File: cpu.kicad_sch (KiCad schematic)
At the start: 41 parts, among them J11 Debug, J12 GPS_Snoop, J13 I2C_Snoop, J6 USB_C_Receptacle_16P, SW1 Reset, U4 STM32H503KBUx, Y1 32768Hz

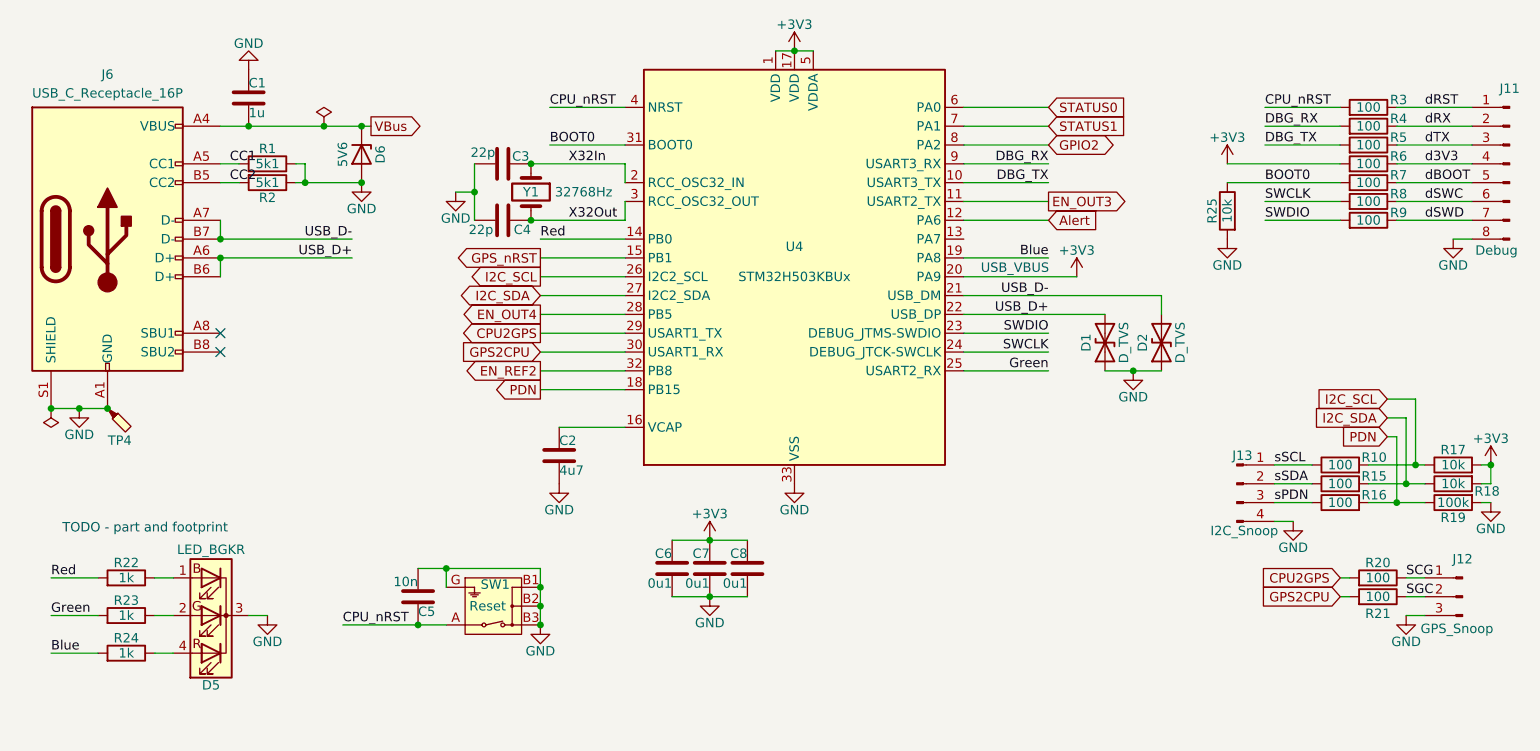
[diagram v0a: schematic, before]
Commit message: Placement looks sane.
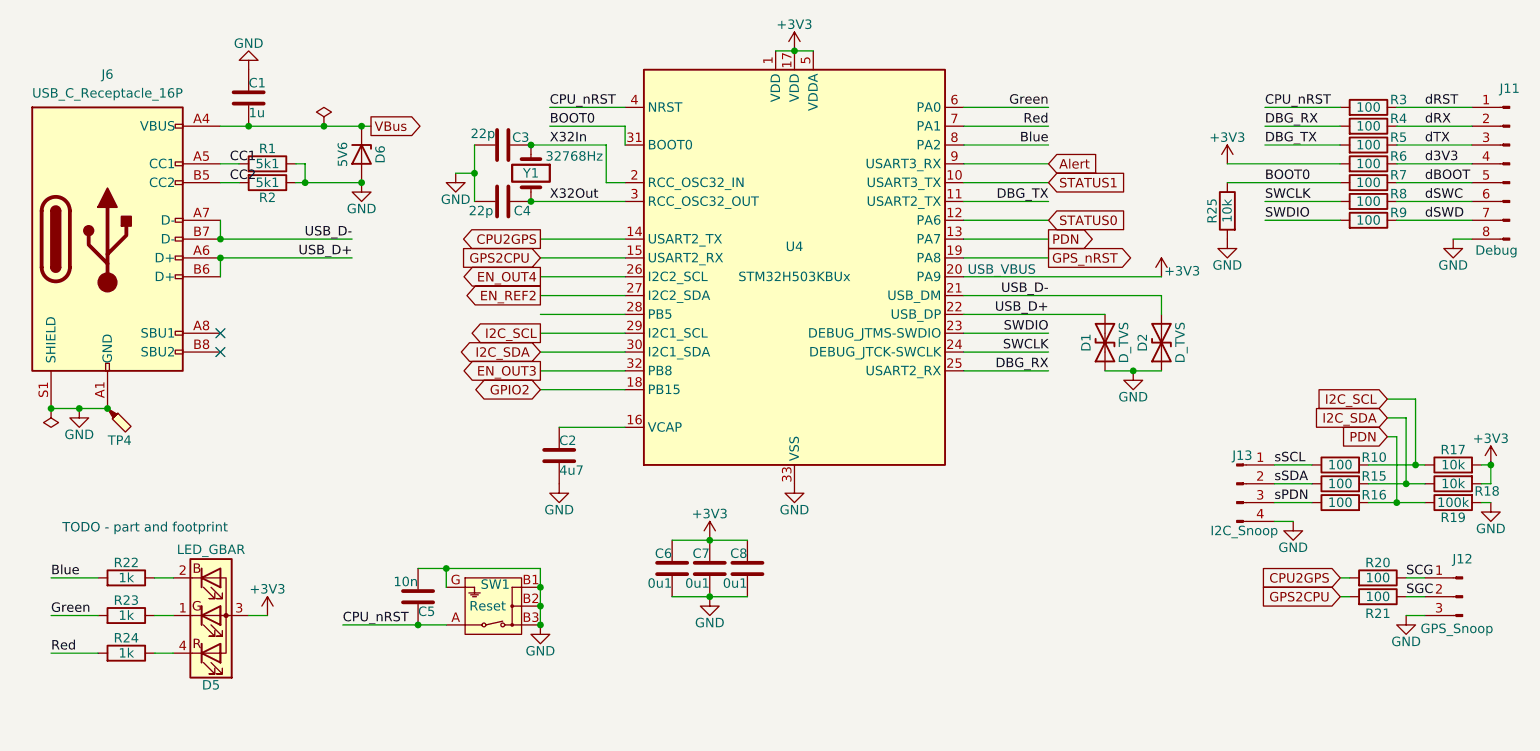
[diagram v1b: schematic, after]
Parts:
- D5: value LED_BGKR -> LED_GBAR; footprint LED_SMD:LED_RGB_Everlight_EASV3015RGBA0_Horizontal -> Parts:LED-QPLB615-RGB; symbol Device:LED_BGKR -> Device:LED_GBAR
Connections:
- net +3V3: now also D5.3 (A)
- net Alert: now also U4.9 (PA3); no longer U4.12 (PA6)
- net Blue: now also R22.2, U4.8 (PA2); no longer R24.2, U4.19 (PA8)
- net CPU2GPS: now also U4.14 (PB0); no longer U4.29 (PB6)
- net DBG_RX: now also U4.25 (PA15(JTDI)); no longer U4.9 (PA3)
- net DBG_TX: now also U4.11 (PA5); no longer U4.10 (PA4)
- net EN_OUT3: now also U4.32 (PB8); no longer U4.11 (PA5)
- net EN_OUT4: now also U4.26 (PB3(JTDO); no longer U4.28 (PB5)
- net EN_REF2: now also U4.27 (PB4(NJTRST)); no longer U4.32 (PB8)
- net GND: no longer D5.3 (K)
- net GPIO2: now also U4.18 (PB15); no longer U4.8 (PA2)
- net GPS2CPU: now also U4.15 (PB1); no longer U4.30 (PB7)
- net GPS_nRST: now also U4.19 (PA8); no longer U4.15 (PB1)
- net Green: now also U4.6 (PA0); no longer U4.25 (PA15(JTDI))
- net I2C_SCL: now also U4.29 (PB6); no longer U4.26 (PB3(JTDO)
- net I2C_SDA: now also U4.30 (PB7); no longer U4.27 (PB4(NJTRST))
- net PDN: now also U4.13 (PA7); no longer U4.18 (PB15)
- net Red: now also R24.2, U4.7 (PA1); no longer R22.2, U4.14 (PB0)
- net STATUS0: now also U4.12 (PA6); no longer U4.6 (PA0)
- net STATUS1: now also U4.10 (PA4); no longer U4.7 (PA1)
- net at D5.1 (GK): now also R23.1; no longer R22.1
- net at D5.2 (BK): now also R22.1; no longer R23.1
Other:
- moved on the sheet: C3, C4, D5, Y1

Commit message: Routing well underway
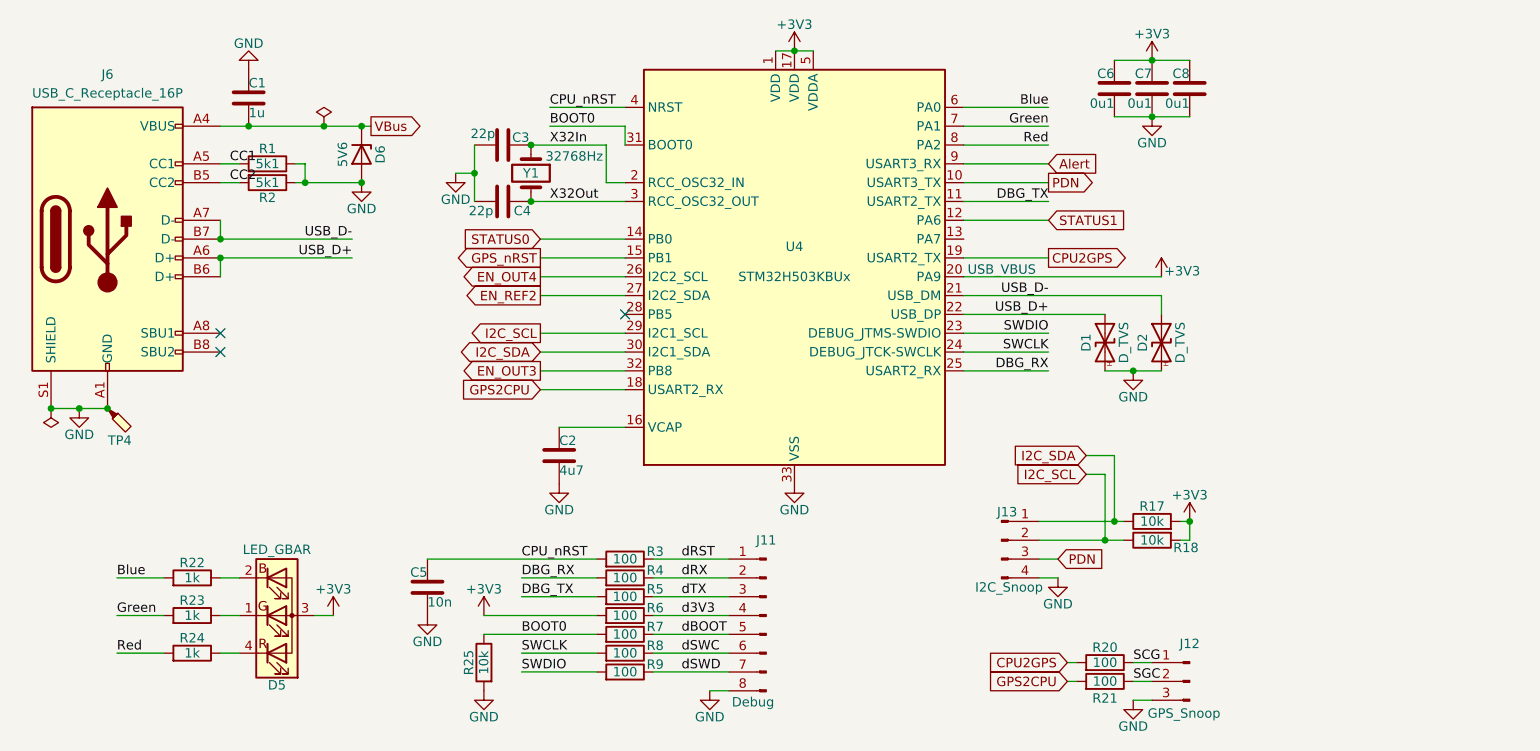
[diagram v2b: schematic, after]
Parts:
- removed R10, R15, R16: 100, Resistor_SMD:R_0402_1005Metric, symbol Device:R
- removed R19: 100k, Resistor_SMD:R_0402_1005Metric, symbol Device:R
- removed SW1: Reset, Parts:SOU-242HNT_MIT, symbol Parts:SOU-242HNT
- D1, D2: footprint Diode_SMD:D_0402_1005Metric_Pad0.77x0.64mm_HandSolder -> Parts:HHS_0402; symbol Device:D_TVS -> Parts:D_TVS; now in the parts list
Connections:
- net GPIO2 is gone; now on net GPS2CPU: U4.18 (PB15)
- net sPDN is gone; now on net PDN: J13.3 (Pin_3)
- net sSCL is gone; now on net I2C_SDA: J13.1 (Pin_1)
- net sSDA is gone; now on net I2C_SCL: J13.2 (Pin_2)
- net Blue: now also U4.6 (PA0); no longer U4.8 (PA2)
- net CPU2GPS: now also U4.19 (PA8); no longer U4.14 (PB0)
- net GND: now also D1.2 (A2), D2.2 (A2); no longer D1.1 (A1), D2.1 (A1)
- net GPS2CPU: no longer U4.15 (PB1)
- net GPS_nRST: now also U4.15 (PB1); no longer U4.19 (PA8)
- net Green: now also U4.7 (PA1); no longer U4.6 (PA0)
- net I2C_SCL: now also R18.1; no longer R17.1
- net I2C_SDA: now also R17.1; no longer R18.1
- net PDN: now also U4.10 (PA4); no longer U4.13 (PA7)
- net Red: now also U4.8 (PA2); no longer U4.7 (PA1)
- net STATUS0: now also U4.14 (PB0); no longer U4.12 (PA6)
- net STATUS1: now also U4.12 (PA6); no longer U4.10 (PA4)
- net USB_D+: now also D1.1 (A1); no longer D1.2 (A2)
- net USB_D-: now also D2.1 (A1); no longer D2.2 (A2)
- no-connect marks 2 -> 3
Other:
- note removed: "TODO - part and footprint"
- moved on the sheet: C5, C6, C7, C8, D5, J11, J12, J13, R17, R18, R20, R21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
